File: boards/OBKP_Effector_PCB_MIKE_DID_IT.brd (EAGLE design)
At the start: 66.9 x 57.9 mm, 34 parts

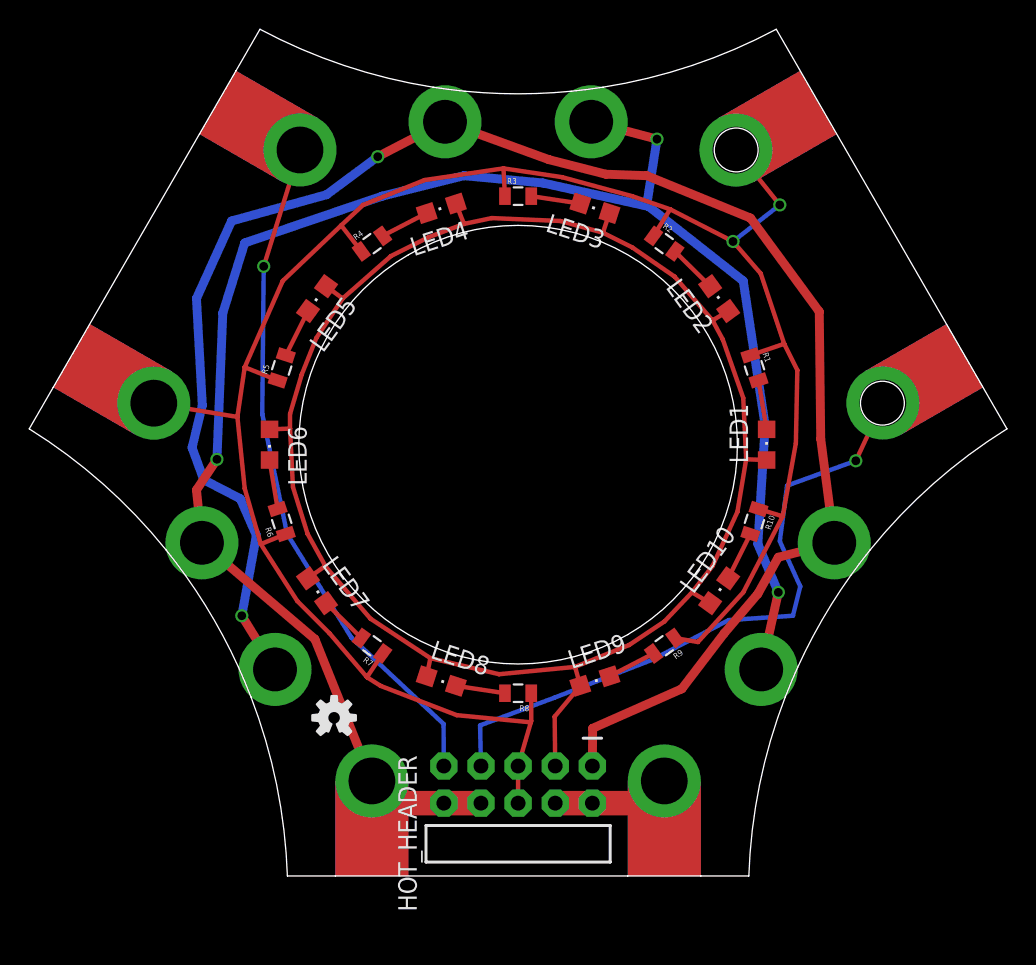
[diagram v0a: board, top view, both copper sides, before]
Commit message: cleaned up board
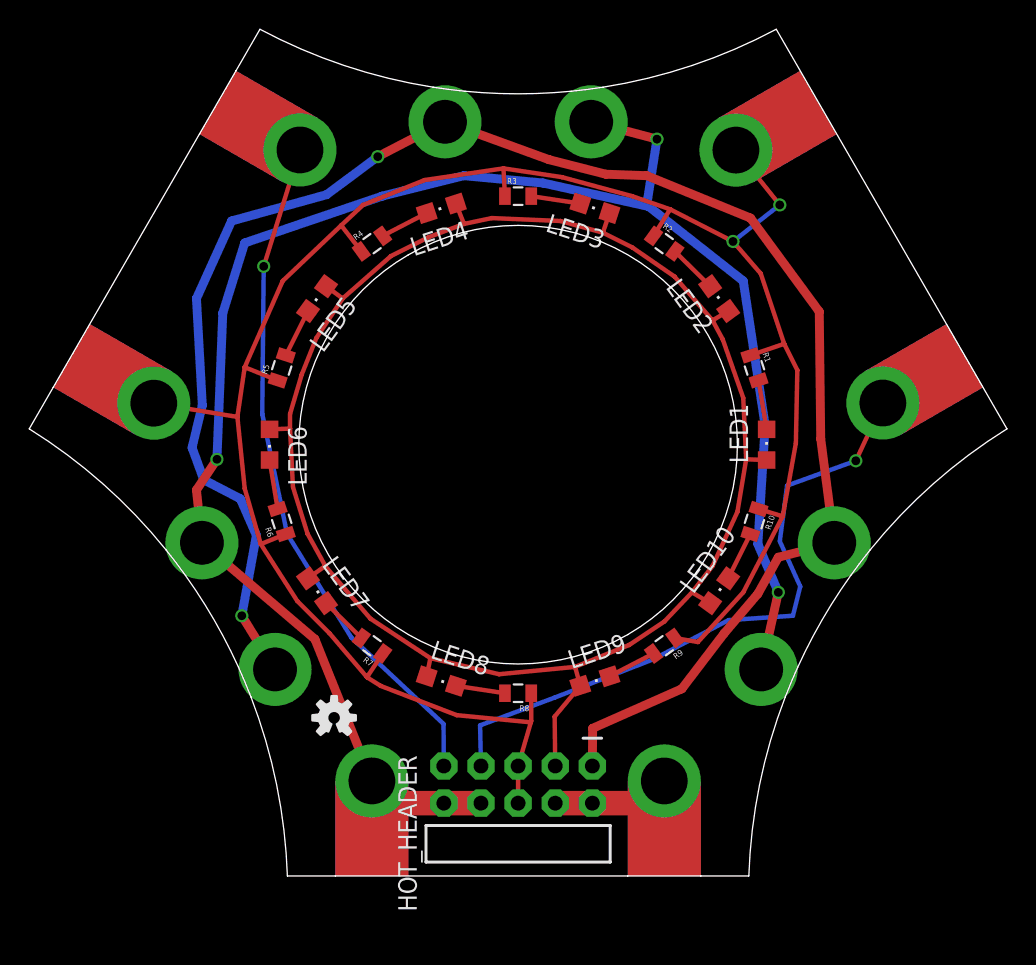
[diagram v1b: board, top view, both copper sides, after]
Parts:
- moved FAN_0_PWM 39.2 mm to (28.0, 51.1), turned to 0 degrees
- moved FAN_1_PWM 39.2 mm to (54.6, 22.3), turned to 330 degrees
- renumbered FAN_0_VCC to FAN_0_12V, FAN_1_VCC to FAN_1_12V, FAN_2_VCC to FAN_2_12V, HOT_VCC to HOT_12V, PROBE+ to PROBE_SIG, PROBE- to PROBE_GND, THERM+ to THERM_SIG, THERM- to THERM_GND
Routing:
- net N$15: track 13.6 -> 10.4 mm
